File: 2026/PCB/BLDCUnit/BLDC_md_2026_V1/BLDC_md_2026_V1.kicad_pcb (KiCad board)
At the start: 2 copper layers, 40 x 51 mm, 86 parts, among them J1 Conn_01x07_Pin, J2 Conn_01x02_Pin, J3 Conn_01x03_Socket, J4 Conn_01x02_Socket, J5 Conn_01x06_Socket, SW1 SW_MEC_5E, SW2 SW_MEC_5E, U1 MAX3051

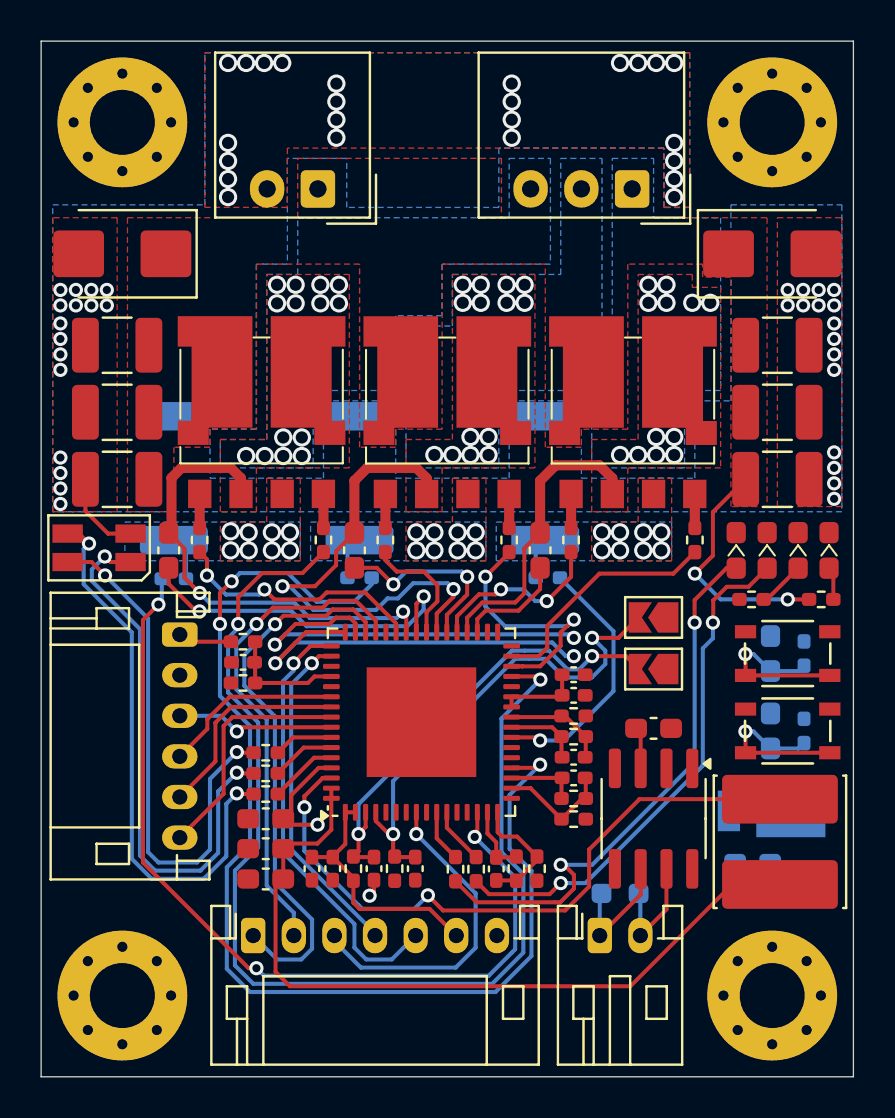
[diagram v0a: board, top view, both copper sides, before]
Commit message: 配線改良
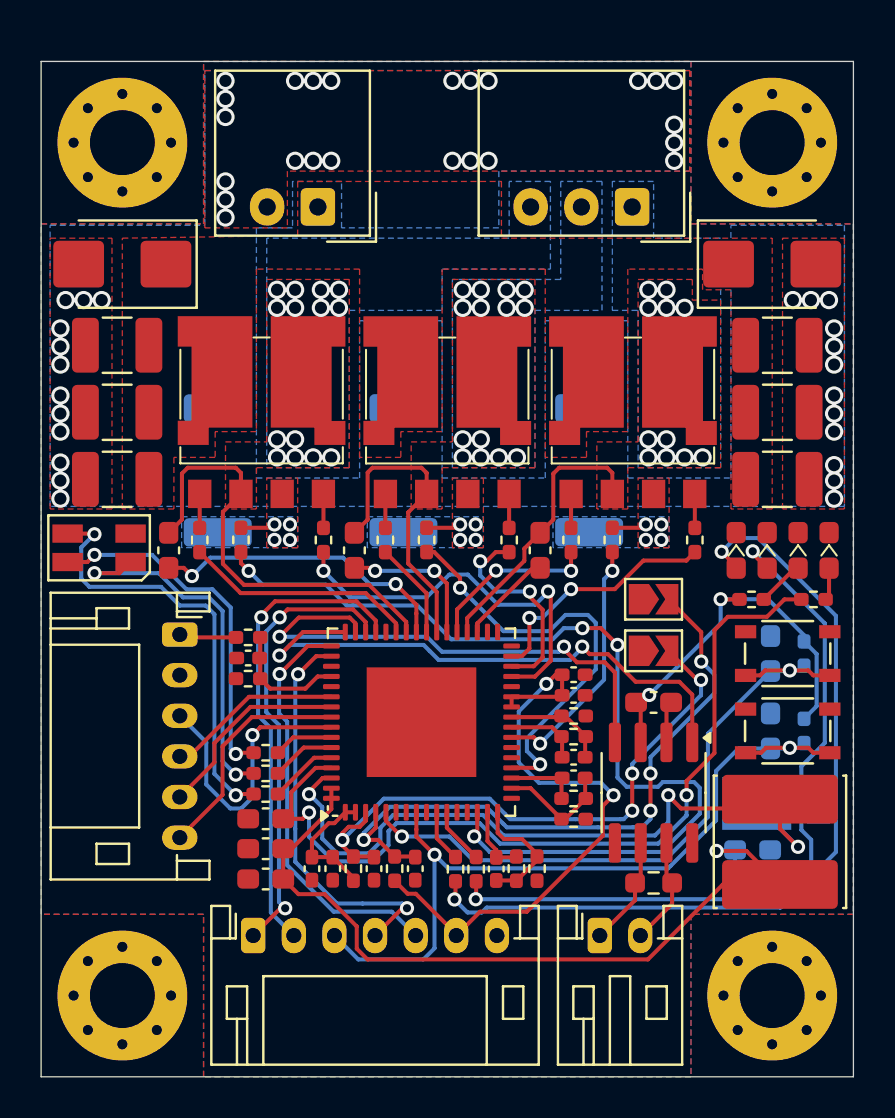
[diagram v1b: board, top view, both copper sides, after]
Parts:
- R21, R22, R27, R32: moved to F.Cu
- moved R32 3.82 mm to (209.8, 74.6), turned to -90 degrees
- moved R27 3.79 mm to (219.0, 74.6), turned to -90 degrees
- moved R22 3.68 mm to (228.1, 74.6), turned to -90 degrees
- moved R18 2.19 mm to (227.0, 71.1)
- moved R19 2.19 mm to (217.8, 71.1)
- moved R20 2.19 mm to (208.7, 71.1)
- moved R21 1.73 mm to (230.2, 91.5)
- moved C21 1.28 mm to (230.2, 82.6)
- moved U1 1.28 mm to (230.2, 87.0)
- moved REF** 1.00 mm to (236.0, 55.0)
- moved REF** 1.00 mm to (204.0, 55.0)
- moved JP1 0.90 mm to (230.2, 80.0), turned to 0 degrees
- moved JP2 0.90 mm to (230.2, 77.5), turned to 0 degrees
- moved J2 0.89 mm to (213.6, 58.2)
- moved J3 0.89 mm to (229.1, 58.2)
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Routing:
- net +3V3: track 21.5 -> 58.9 mm, vias 0 -> 4
- net GLS1: track 56.2 -> 19.6 mm
- net OP2_VINP: track 56.9 -> 20.8 mm, vias 3 -> 2
- net +50V: track 17.5 -> 42.4 mm, vias 3 -> 2
- net USW: track 8.55 -> 32.5 mm, vias 1 -> 2
- net NRST: track 24.6 -> 39.5 mm
- net Net-(D5-A): track 27.4 -> 41.4 mm
- net Net-(D6-A): track 25.7 -> 36.9 mm
- net Net-(D2-BA): track 26.8 -> 17.5 mm
- net BLDC_V: track 24.5 -> 15.1 mm, vias 16 -> 14
- net Net-(D2-GA): track 27.5 -> 18.3 mm
- net JP2: track 24.2 -> 33.1 mm, vias 2 -> 4
- net CAN_TX: track 19.5 -> 28.2 mm
- net JP1: track 22.8 -> 30.0 mm, vias 2 -> 4
- net Net-(D2-RA): track 27.5 -> 21.3 mm
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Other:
- board size 40 x 51 mm -> 40 x 50 mm

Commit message: 配線完了
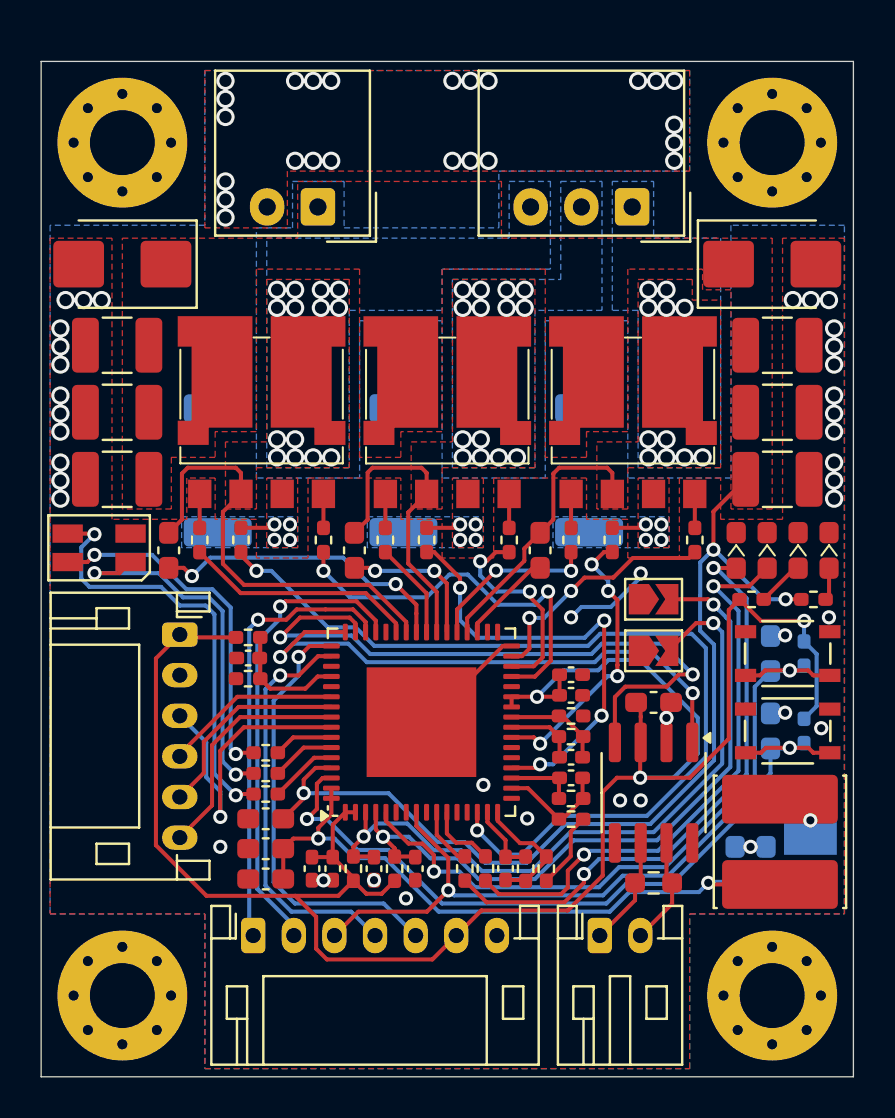
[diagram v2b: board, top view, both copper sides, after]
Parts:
- moved D1 2.46 mm to (237.9, 89.4), turned to -90 degrees
- moved C12 1.12 mm to (234.2, 90.5), turned to 90 degrees
- moved C11 1.01 mm to (235.7, 90.5), turned to 90 degrees
- moved R10 0.46 mm to (220.9, 90.7)
- moved R11 0.46 mm to (221.9, 90.7)
- moved C27 0.46 mm to (222.9, 90.7)
- moved R33 0.46 mm to (224.9, 90.8)
- moved R36 0.46 mm to (223.9, 90.8)
- moved C25 0.13 mm to (226.1, 85.3)
- moved C26 0.13 mm to (226.1, 86.3)
- moved C3 0.13 mm to (226.1, 81.2)
- moved C4 0.13 mm to (226.1, 82.2)
- moved R23 0.13 mm to (226.1, 83.2)
- moved R26 0.13 mm to (226.1, 84.2)
- moved R28 0.13 mm to (226.1, 88.3)
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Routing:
- net +3V3: track 58.9 -> 102.6 mm, vias 4 -> 3
- net GND: track 2.06 -> 18.1 mm, vias 48 -> 64
- net Net-(D5-A): track 41.4 -> 29.2 mm
- net Net-(D6-A): track 36.9 -> 28.4 mm
- net CAN_RX: track 25.6 -> 32.8 mm
- net +50V: track 42.4 -> 48.4 mm, vias 2 -> 3
- net +8V: track 40.3 -> 34.4 mm, vias 1 -> 2
- net JP1: track 30.0 -> 34.4 mm, vias 4 -> 2
- net Net-(D1-K): track 36.2 -> 32.9 mm, vias 3 -> 2
- net NRST: track 39.5 -> 36.8 mm
- net USW: track 32.5 -> 34.3 mm
- net OP3_VINP: track 12.4 -> 14.0 mm, vias 2 -> 4
- net OP1_VINP: track 46.9 -> 45.5 mm, vias 4 -> 2
- net OP2_VINP: track 20.8 -> 22.3 mm, vias 2 -> 4
- net JP2: track 33.1 -> 34.5 mm, vias 4 -> 2
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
